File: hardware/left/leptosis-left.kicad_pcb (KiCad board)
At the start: 4 copper layers, 93.5 x 72.3 mm, 91 parts, among them J1 USB_C_Receptacle_USB2.0_14P, J2 Conn_01x02, Q2 2N7002, SW10 SW_Push, SW11 SW_Push, SW12 SW_Push, SW14 SW_Push, SW15 SW_Push, SW16 SW_Push, SW17 SW_Push, SW18 SW_Push, SW2 SW_Push, SW22 SW_Push, SW23 SW_Push, SW24 SW_Push, SW3 SW_Push, SW31 SW_SPDT, SW4 SW_Push, SW5 SW_Push, SW6 SW_Push, SW8 SW_Push, SW9 SW_Push, U1 nRF52840, U2 BQ24075RGT, U3 MAX17048X, Y1 32MHz 12pF, Y2 32.768kHz 12.5pF

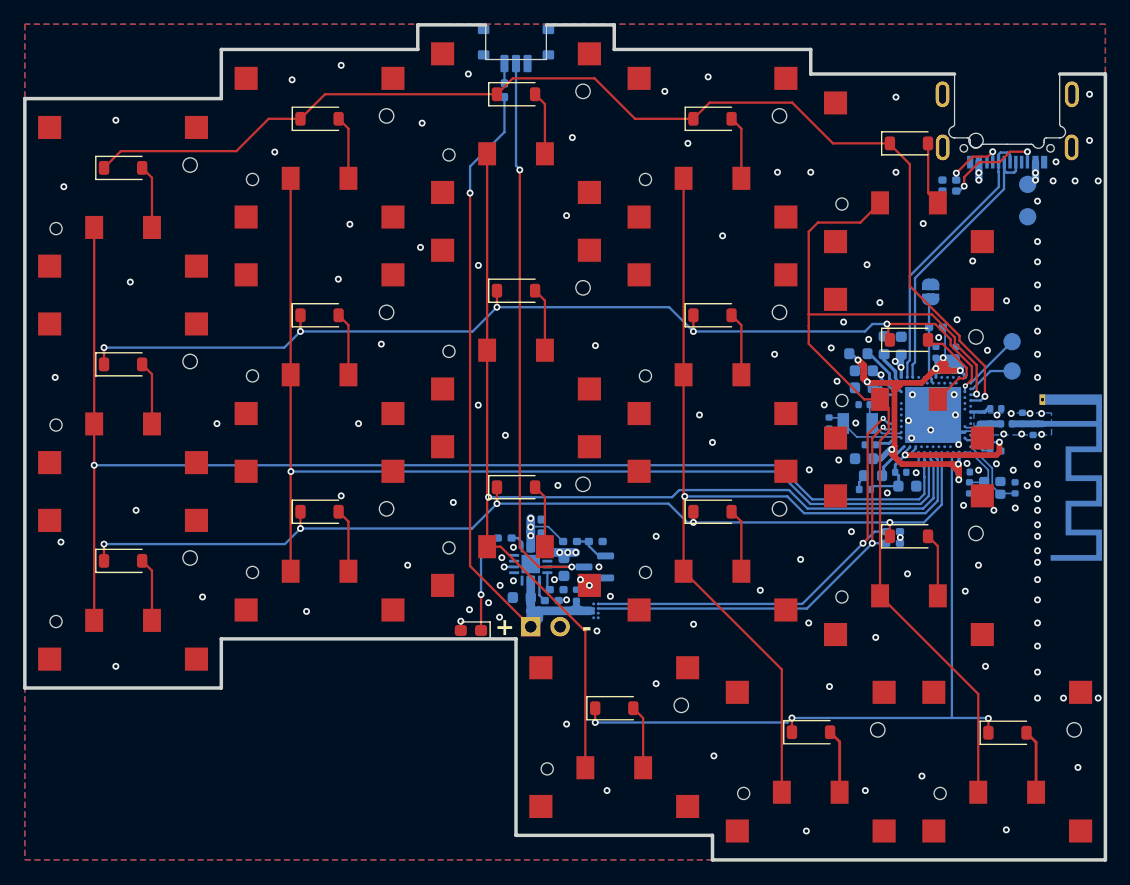
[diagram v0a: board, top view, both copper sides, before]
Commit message: Finish
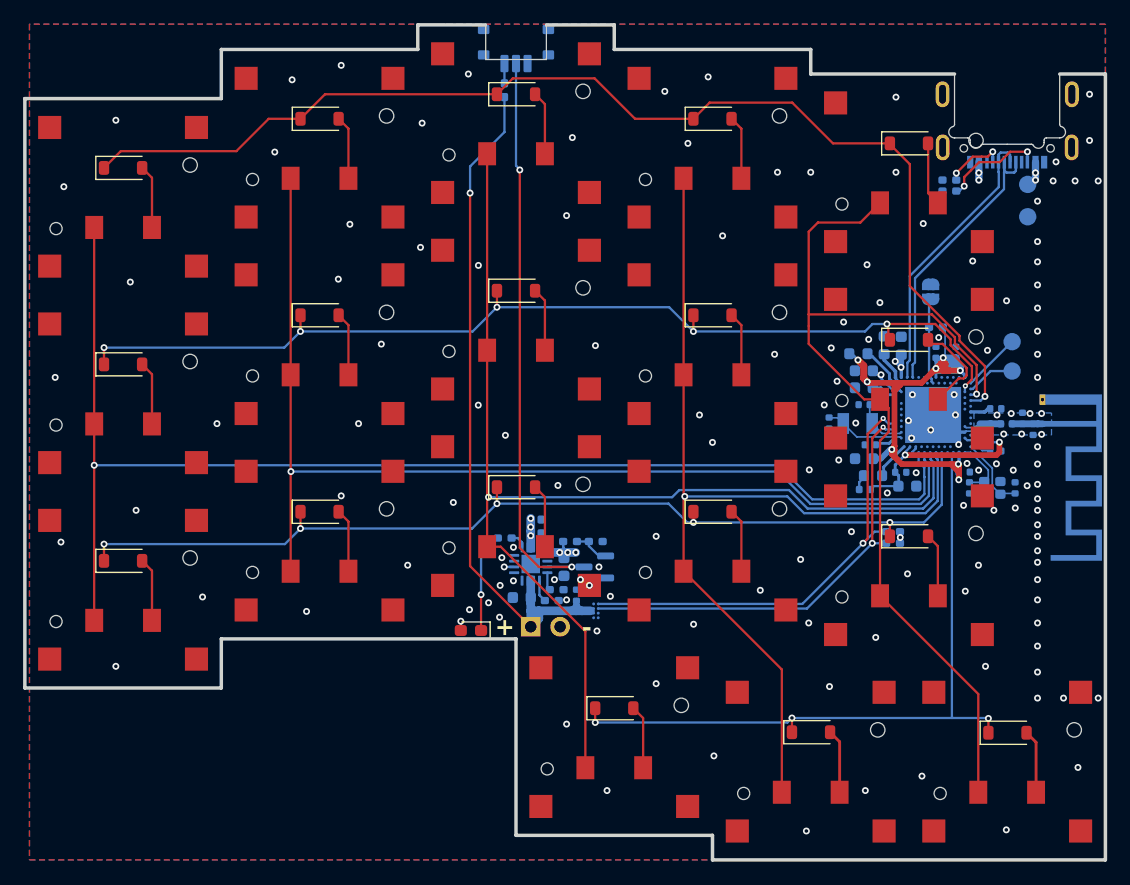
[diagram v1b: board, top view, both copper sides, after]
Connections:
- R7 pad 2: +5V -> VBUS
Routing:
- net +5V: track 12.0 -> 8.74 mm
- net VBUS: track 8.29 -> 11.1 mm
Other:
- board text removed: "301540 battery or 302025"
